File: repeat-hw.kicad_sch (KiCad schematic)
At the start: 0 parts

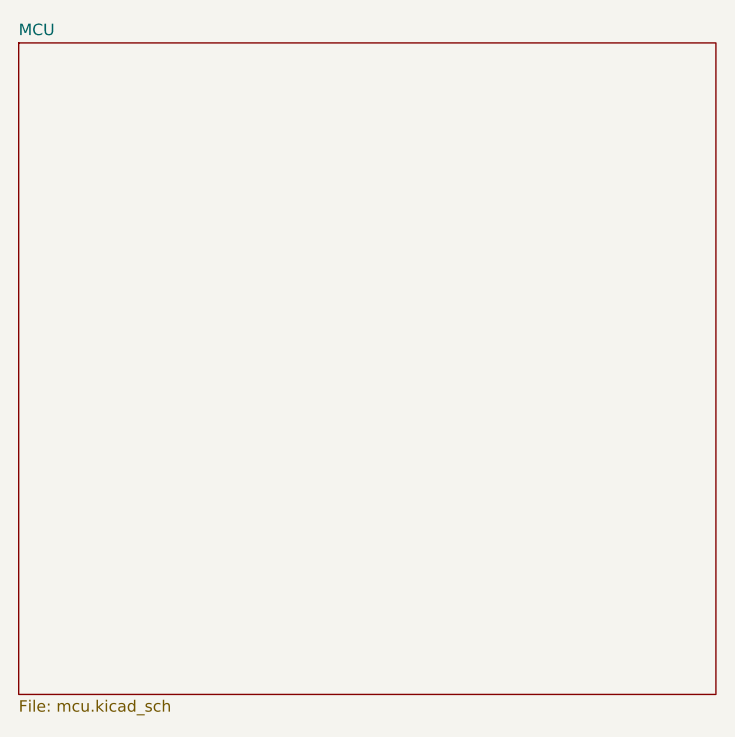
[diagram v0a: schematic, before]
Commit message: added W5100
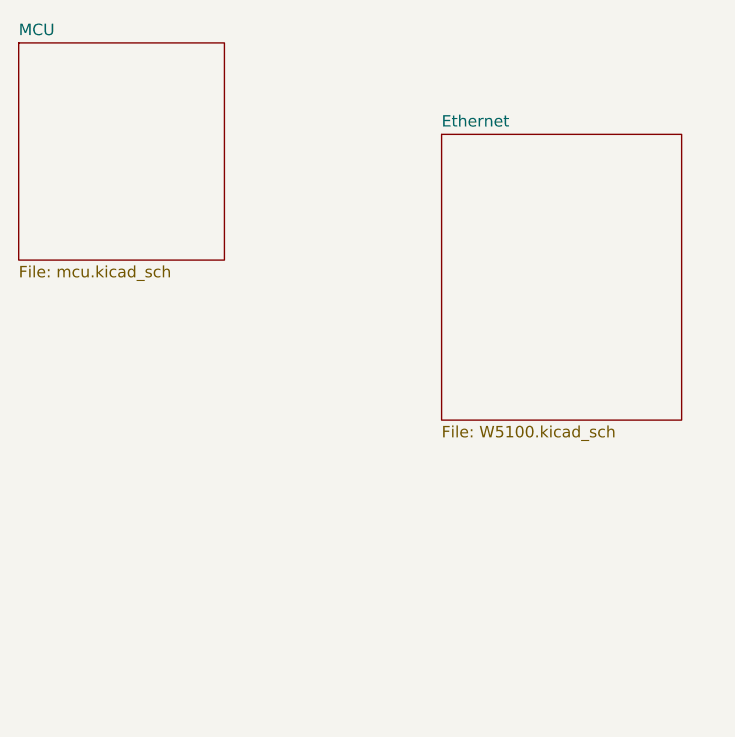
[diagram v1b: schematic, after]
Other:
- added sheet Ethernet (W5100.kicad_sch)
